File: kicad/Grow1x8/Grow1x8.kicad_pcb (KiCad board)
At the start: 2 copper layers, 77 x 24.5 mm, 3 parts, among them J1 Screw_Terminal_01x02, J2 Screw_Terminal_01x02

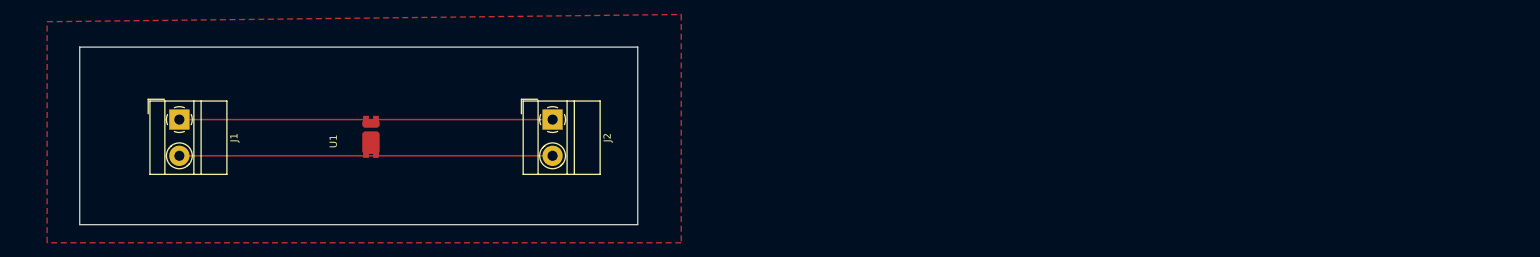
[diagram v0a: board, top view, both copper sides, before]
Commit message: latest
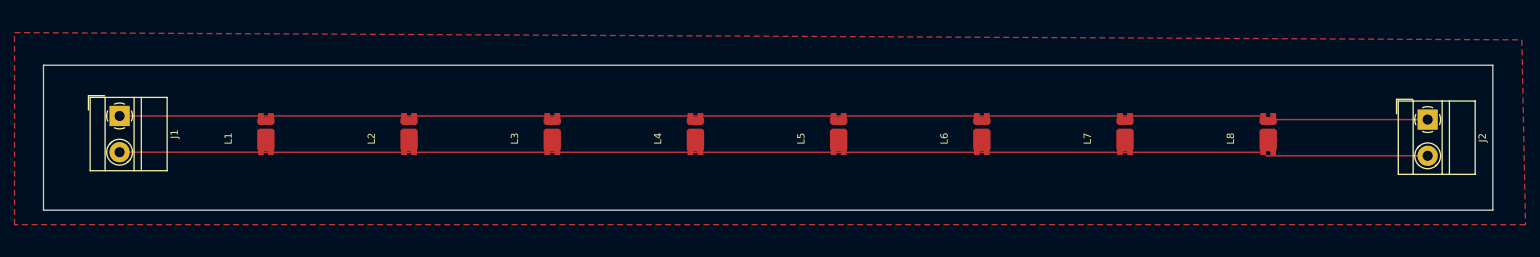
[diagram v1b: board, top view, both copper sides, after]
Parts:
- removed U1: ~, dlaw:LED 5630
- added L1: ~, dlaw:LED 5630, F.Cu at (90.2, 53.8)
- added L2: ~, dlaw:LED 5630, F.Cu at (109.9, 53.8)
- added L3: ~, dlaw:LED 5630, F.Cu at (129.7, 53.8)
- added L4: ~, dlaw:LED 5630, F.Cu at (149.5, 53.8)
- added L5: ~, dlaw:LED 5630, F.Cu at (169.2, 53.8)
- added L6: ~, dlaw:LED 5630, F.Cu at (189.0, 53.8)
- added L7: ~, dlaw:LED 5630, F.Cu at (208.7, 53.8)
- added L8: ~, dlaw:LED 5630, F.Cu at (228.5, 53.8)
- moved J2 120.8 mm to (250.5, 51.0)
- moved J1 8.27 mm to (70.0, 50.5)
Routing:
- net GND: track 51.6 -> 180.7 mm
- net +3.3V: track 51.6 -> 180.7 mm
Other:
- board size 77 x 24.5 mm -> 200 x 20 mm
